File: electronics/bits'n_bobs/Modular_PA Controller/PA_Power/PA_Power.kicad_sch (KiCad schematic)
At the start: 54 parts, among them J1 Screw_Terminal_01x02, J2 Screw_Terminal_01x02, J3 Conn_01x04, J4 Conn_01x04, J5 Conn_01x04, J6 Conn_01x04, J7 Conn_01x02, Q1 Q_PMOS_DGS, Q2 Q_NMOS_DGS, U1 ACS758xCB-050U-PFF, U2 LMR38020, U3 ADS1015IDGS, U4 PCF8574A, U5 MCP4725xxx-xCH, U6 AP2204K-ADJ

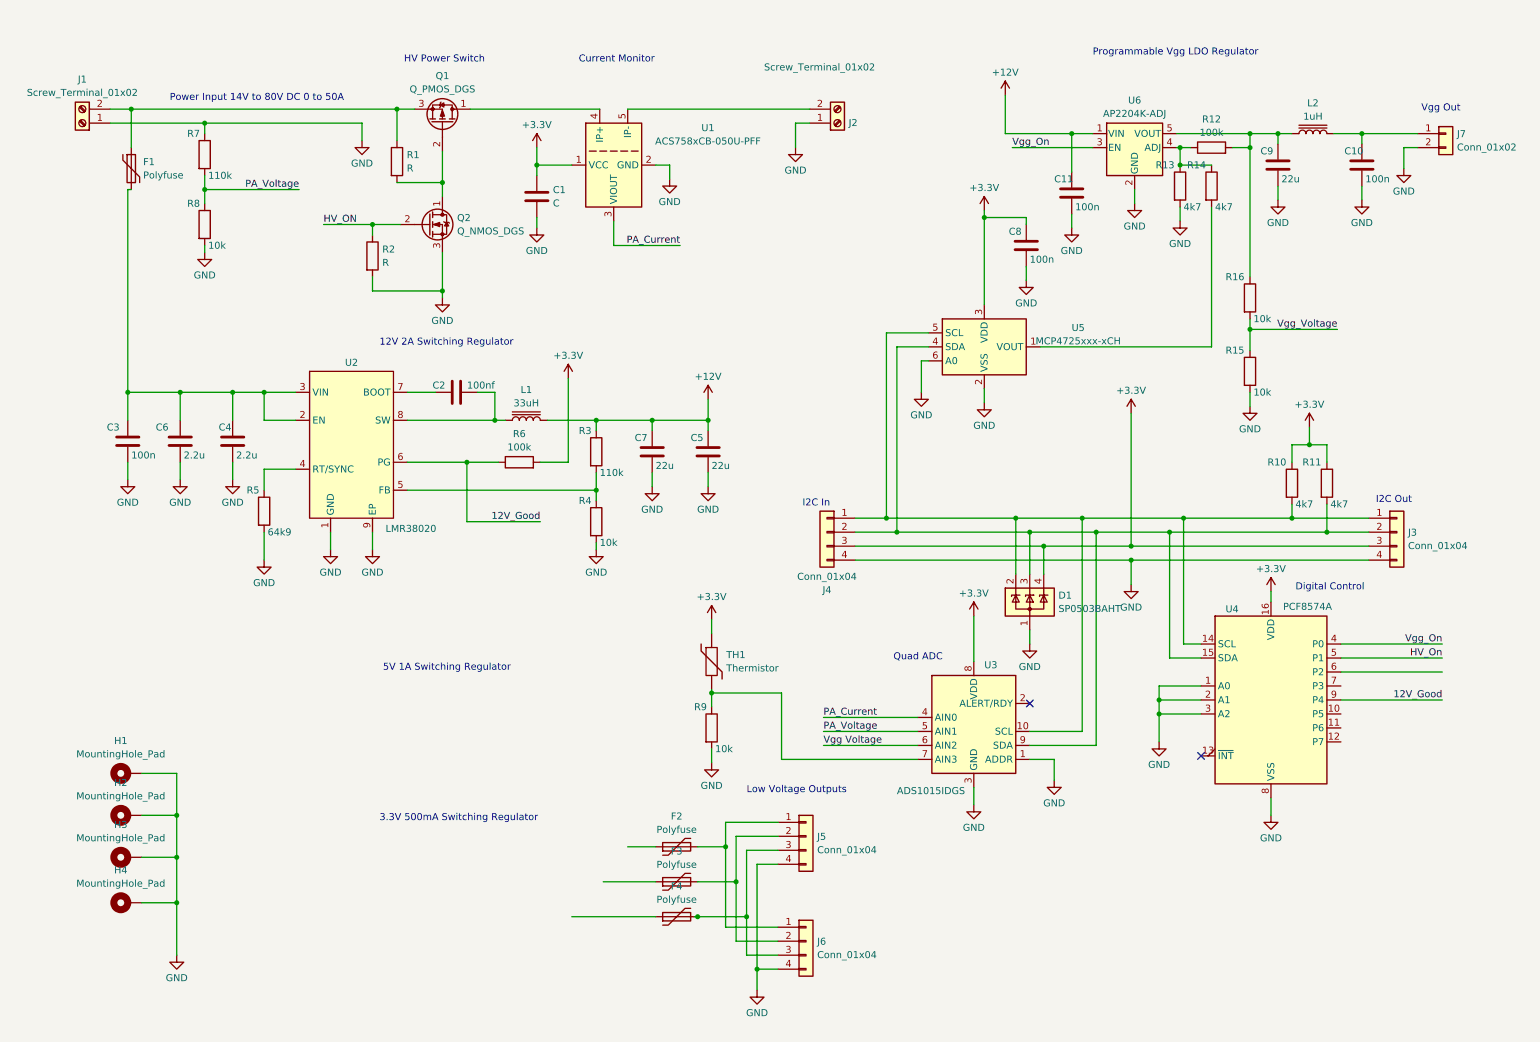
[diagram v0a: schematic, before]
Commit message: Updates in electronics bits and bobs
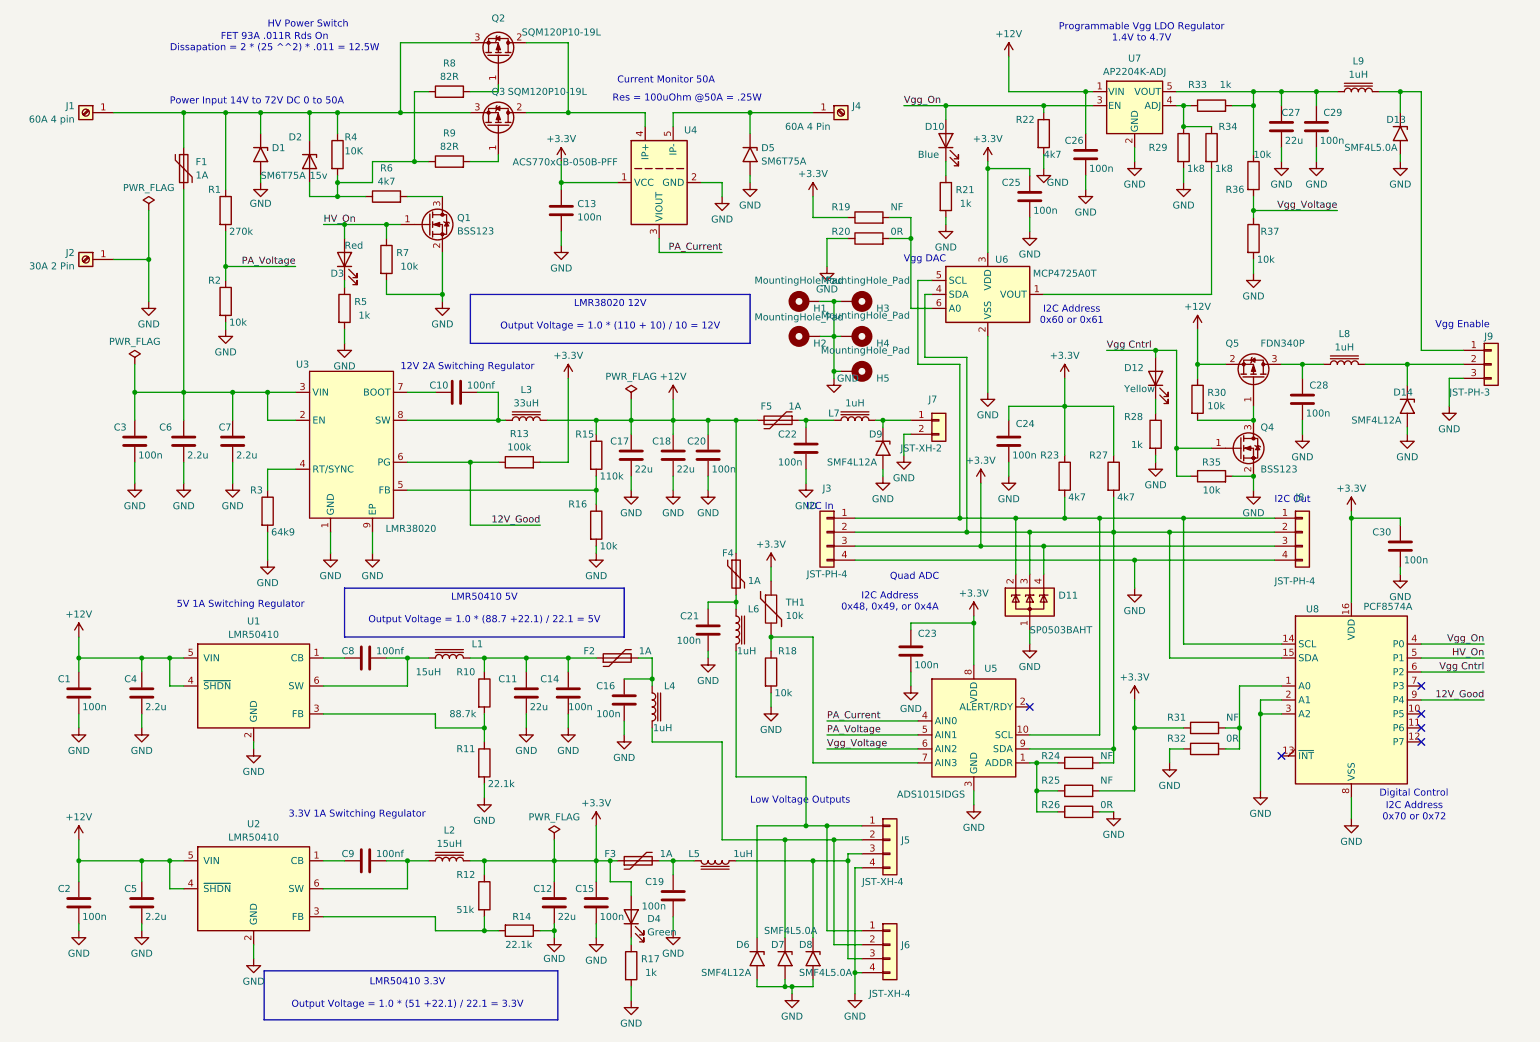
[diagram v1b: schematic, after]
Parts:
- removed J1, J2: Screw_Terminal_01x02, symbol Connector:Screw_Terminal_01x02
- removed U1: ACS758xCB-050U-PFF, Sensor_Current:Allegro_CB_PFF, symbol Sensor_Current:ACS758xCB-050U-PFF
- added C1, C14, C15, C16, C19, C2, C20, C21, C22, C23, C24, C28, C30: 100n, Capacitor_SMD:C_0603_1608Metric, symbol Device:C
- added C11, C12: 22u, Capacitor_SMD:C_1210_3225Metric, symbol Device:C
- added C4, C5: 2.2u, Capacitor_SMD:C_0603_1608Metric, symbol Device:C
- added C8, C9: 100nf, Capacitor_SMD:C_0603_1608Metric, symbol Device:C
- added D1, D5: SM6T75A, Diode_SMD:D_SMB, symbol Diode:SM6T100A
- added D10: Blue, LED_SMD:LED_0603_1608Metric, symbol Device:LED
- added D12: Yellow, LED_SMD:LED_0603_1608Metric, symbol Device:LED
- added D13, D7, D8: SMF4L5.0A, Diode_SMD:D_SOD-123F, symbol Diode:SM6T100A
- added D14, D6, D9: SMF4L12A, Diode_SMD:D_SOD-123F, symbol Diode:SM6T100A
- added D2: 15v, Diode_SMD:Nexperia_CFP3_SOD-123W, symbol Device:D_Zener
- added D3: Red, LED_SMD:LED_0603_1608Metric, symbol Device:LED
- added D4: Green, LED_SMD:LED_0603_1608Metric, symbol Device:LED
- added F5: 1A, Fuse:Fuse_1812_4532Metric, symbol Device:Polyfuse
- added H5: MountingHole_Pad, MountingHole:MountingHole_3.2mm_M3_DIN965_Pad, symbol Mechanical:MountingHole_Pad
- added J1: 60A 4 pin, PA_Control:Fat_Power 4, symbol Connector:Screw_Terminal_01x01
- added J2: 30A 2 Pin, PA_Control:Fat_Power 2, symbol Connector:Screw_Terminal_01x01
- added J4: 60A 4 Pin, PA_Control:Fat_Power 4, symbol Connector:Screw_Terminal_01x01
- added J9: JST-PH-3, Connector_JST:JST_PH_S3B-PH-SM4-TB_1x03-1MP_P2.00mm_Horizontal, symbol Connector_Generic:Conn_01x03
- added L1, L2: 15uH, Inductor_SMD:L_Wuerth_MAPI-4030, symbol Device:L_Iron
- added L4, L5, L6, L7, L8: 1uH, Inductor_SMD:L_0805_2012Metric, symbol Device:L_Iron
- added Q2: SQM120P10-19L, PA_Control:TO263_Heatsink_301, symbol Device:Q_PMOS_GDS
- added Q4: BSS123, Package_TO_SOT_SMD:SOT-23, symbol Transistor_FET:BSS123
- added Q5: FDN340P, Package_TO_SOT_SMD:SOT-23, symbol Transistor_FET:FDN340P
- added R10: 88.7k, Resistor_SMD:R_0603_1608Metric, symbol Device:R
- added R11, R14: 22.1k, Resistor_SMD:R_0603_1608Metric, symbol Device:R
- added R12: 51k, Resistor_SMD:R_0603_1608Metric, symbol Device:R
- added R17, R21, R28, R5: 1k, Resistor_SMD:R_0603_1608Metric, symbol Device:R
- added R19, R24, R25, R31: NF, Resistor_SMD:R_0603_1608Metric, symbol Device:R
- added R20, R26, R32: 0R, Resistor_SMD:R_0603_1608Metric, symbol Device:R
- added R22, R6: 4k7, Resistor_SMD:R_0603_1608Metric, symbol Device:R
- added R30, R35: 10k, Resistor_SMD:R_0603_1608Metric, symbol Device:R
- added R8, R9: 82R, Resistor_SMD:R_0603_1608Metric, symbol Device:R
- added U1, U2: LMR50410, Package_TO_SOT_SMD:SOT-23-6, symbol PA_Control:LMR50410
- added U4: ACS770xCB-050B-PFF, PA_Control:Allegro_CB_PFF, symbol Sensor_Current:ACS770xCB-050B-PFF
- C10: renamed from C2; footprint (none) -> Capacitor_SMD:C_0603_1608Metric
- C13: renamed from C1; value C -> 100n; footprint (none) -> Capacitor_SMD:C_0603_1608Metric
- C17: renamed from C7; footprint (none) -> Capacitor_SMD:C_1210_3225Metric
- C18: renamed from C5; footprint (none) -> Capacitor_SMD:C_1210_3225Metric
- C25: renamed from C8; footprint (none) -> Capacitor_SMD:C_0603_1608Metric
- C26: renamed from C11; footprint (none) -> Capacitor_SMD:C_0603_1608Metric
- C27: renamed from C9; footprint (none) -> Capacitor_SMD:C_0805_2012Metric
- C29: renamed from C10; footprint (none) -> Capacitor_SMD:C_0603_1608Metric
- C3: footprint (none) -> Capacitor_SMD:C_0805_2012Metric
- C6: footprint (none) -> Capacitor_SMD:C_1210_3225Metric
- C7: renamed from C4; footprint (none) -> Capacitor_SMD:C_1210_3225Metric
- F1: value Polyfuse -> 1A; footprint (none) -> Fuse:Fuse_Schurter_UMZ250
- F2: renamed from F3; value Polyfuse -> 1A; footprint (none) -> Fuse:Fuse_1812_4532Metric
- F3: renamed from F4; value Polyfuse -> 1A; footprint (none) -> Fuse:Fuse_1812_4532Metric
- F4: renamed from F2; value Polyfuse -> 1A; footprint (none) -> Fuse:Fuse_1812_4532Metric
- H1: renamed from H3; footprint (none) -> MountingHole:MountingHole_3.2mm_M3_DIN965_Pad
- H2: renamed from H4; footprint (none) -> MountingHole:MountingHole_3.2mm_M3_DIN965_Pad
- H3: renamed from H1; footprint (none) -> MountingHole:MountingHole_3.2mm_M3_DIN965_Pad
- H4: renamed from H2; footprint (none) -> MountingHole:MountingHole_3.2mm_M3_DIN965_Pad
- J3: renamed from J4; value Conn_01x04 -> JST-PH-4; footprint (none) -> Connector_JST:JST_PH_B4B-PH-SM4-TB_1x04-1MP_P2.00mm_Vertical
- J5, J6: value Conn_01x04 -> JST-XH-4; footprint (none) -> Connector_JST:JST_XH_S4B-XH-A_1x04_P2.50mm_Horizontal
- J7: value Conn_01x02 -> JST-XH-2; footprint (none) -> Connector_JST:JST_XH_S2B-XH-A_1x02_P2.50mm_Horizontal
- J8: renamed from J3; value Conn_01x04 -> JST-PH-4; footprint (none) -> Connector_JST:JST_PH_B4B-PH-SM4-TB_1x04-1MP_P2.00mm_Vertical
- L3: renamed from L1; footprint (none) -> Inductor_SMD:L_Coilcraft_MSS1210-XXX
- L9: renamed from L2; footprint (none) -> Inductor_SMD:L_0805_2012Metric
- Q1: renamed from Q2; value Q_NMOS_DGS -> BSS123; footprint (none) -> Package_TO_SOT_SMD:SOT-23; symbol Device:Q_NMOS_DGS -> Transistor_FET:BSS123
- Q3: renamed from Q1; value Q_PMOS_DGS -> SQM120P10-19L; footprint (none) -> PA_Control:TO263_Heatsink_301; symbol Device:Q_PMOS_DGS -> Device:Q_PMOS_GDS
- R1: renamed from R7; value 110k -> 270k; footprint (none) -> Resistor_SMD:R_0603_1608Metric
- R13: renamed from R6; footprint (none) -> Resistor_SMD:R_0603_1608Metric
- R15: renamed from R3; footprint (none) -> Resistor_SMD:R_0603_1608Metric
- R16: renamed from R4; footprint (none) -> Resistor_SMD:R_0603_1608Metric
- R18: renamed from R9; footprint (none) -> Resistor_SMD:R_0603_1608Metric
- R2: renamed from R8; footprint (none) -> Resistor_SMD:R_0603_1608Metric
- R23: renamed from R10; footprint (none) -> Resistor_SMD:R_0603_1608Metric
- R27: renamed from R11; footprint (none) -> Resistor_SMD:R_0603_1608Metric
- R29: renamed from R13; value 4k7 -> 1k8; footprint (none) -> Resistor_SMD:R_0603_1608Metric
- R3: renamed from R5; footprint (none) -> Resistor_SMD:R_0603_1608Metric
- R33: renamed from R12; value 100k -> 1k; footprint (none) -> Resistor_SMD:R_0603_1608Metric
- R34: renamed from R14; value 4k7 -> 1k8; footprint (none) -> Resistor_SMD:R_0603_1608Metric
- R36: renamed from R16; footprint (none) -> Resistor_SMD:R_0603_1608Metric
- R37: renamed from R15; footprint (none) -> Resistor_SMD:R_0603_1608Metric
- R4: renamed from R1; value R -> 10K; footprint (none) -> Resistor_SMD:R_0603_1608Metric
- R7: renamed from R2; value R -> 10k; footprint (none) -> Resistor_SMD:R_0603_1608Metric
- TH1: value Thermistor -> 10k; footprint (none) -> Resistor_SMD:R_0603_1608Metric
- U3: renamed from U2; footprint (none) -> PA_Control:lmr38012
- U6: renamed from U5; value MCP4725xxx-xCH -> MCP4725A0T
- U8: renamed from U4; footprint (none) -> Package_SO:SOIC-16W_7.5x10.3mm_P1.27mm
- renumbered D1 to D11, U3 to U5, U6 to U7
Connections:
- net Vgg Voltage is gone; now on net Vgg_Voltage: U5.6 (AIN2)
- net +12V: now also F4.1, C1.1, C2.1, C20.1, C4.1, C5.1, F5.2, Q5.2 (S), R30.1, U1.4 (~{SHDN}), U1.5 (VIN), U2.4 (~{SHDN}), U2.5 (VIN)
- net +3.3V: now also F3.1, C12.1, C15.1, C23.1, C24.1, C30.1, D4.2 (A), L2.2, R12.1, R19.1, R25.2, R31.1, U4.1 (VCC)
- net GND: now also Q1.2 (S), C1.2, C11.2, C12.2, C14.2, C15.2, C16.2, C19.2, C2.2, C20.2, C21.2, C22.2, C23.2, C24.2, C28.2, C30.2, C4.2, C5.2, D1.2 (A2), D13.2 (A2), D14.2 (A2), D5.2 (A2), D6.2 (A2), D7.2 (A2), D8.2 (A2), D9.2 (A2), H5.1, J2.1 (Pin_1), J9.3 (Pin_3), Q4.2 (S), R11.2, R14.1, R17.2, R20.1, R21.2, R22.2, R26.2, R28.2, R32.1, R35.2, R5.2, U1.2 (GND), U2.2 (GND), U4.2 (GND); no longer Q1.3 (S), R1.1, U5.1 (ADDR), U6.6 (A0), U8.1 (A0)
- net HV_On: now also Q1.1 (G), R7.1, D3.2 (A)
- net PA_Current: now also U4.3 (VIOUT)
- net Vgg_On: now also D10.2 (A), R22.1
- net at C27.1, L9.1, R33.2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: now also C29.1
- net at J5.1 (Pin_1), J6.1 (Pin_1): now also D6.1 (A1), L6.2; no longer F4.2
- net at D11.3 (K), J3.2 (Pin_2), J8.2 (Pin_2)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: now also R24.2
- net at F2.1: now also C11.1, C14.1, L1.2, R10.1
- net at J5.2 (Pin_2), J6.2 (Pin_2): now also D7.1 (A1), L4.2; no longer F2.2
- net at F1.1, Q3.3 (S), R4.1: now also R1.1, D1.1 (A1), D2.1 (K), J1.1 (Pin_1), Q2.3 (S)
- net Vgg Cntrl: now reaches U8.6 (P2)
- net Vgg Cntrl: now also D12.2 (A), Q4.1 (G), R35.1
- net at J5.3 (Pin_3), J6.3 (Pin_3): now also D8.1 (A1), L5.1; no longer F3.2
- net at Q3.1 (G): now also R9.2
- removed net HV_ON: Q1.2 (G), R7.1
- new net: C21.1, F4.2, L6.1
- new net: R24.1, R25.1, R26.1, U5.1 (ADDR)
- new net: R19.2, R20.2, U6.6 (A0)
- new net: Q4.3 (D), Q5.1 (G), R30.2
- new net: C16.1, F2.2, L4.1
- new net: C8.2, L1.1, U1.6 (SW)
- new net: D2.2 (A), R4.2, R6.1, R8.1, R9.1
- new net: D9.1 (A1), J7.1 (Pin_1), L7.2
- new net: D3.1 (K), R5.1
- new net: C22.1, F5.1, L7.1
- new net: R12.2, R14.2, U2.3 (FB)
- new net: D14.1 (A1), J9.2 (Pin_2), L8.2
- new net: D13.1 (A1), J9.1 (Pin_1), L9.2
- new net: C8.1, U1.1 (CB)
- new net: C9.2, L2.1, U2.6 (SW)
- new net: C28.1, L8.1, Q5.3 (D)
- new net: D5.1 (A1), J4.1 (Pin_1), U4.5 (IP-)
- new net: D4.1 (K), R17.1
- new net: C9.1, U2.1 (CB)
- new net: Q2.2 (D), Q3.2 (D), U4.4 (IP+)
- new net: R31.2, R32.2, U8.1 (A0)
- new net: D12.1 (K), R28.1
- new net: C19.1, F3.2, L5.2
- new net: Q2.1 (G), R8.2
- new net: R10.2, R11.1, U1.3 (FB)
- new net: Q1.3 (D), R6.2
- new net: D10.1 (K), R21.1
- no-connect marks 2 -> 6
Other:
- note added: "3.3V 1A Switching Regulator"
- note added: "Current Monitor 50A"
- note added: "FET 93A .011R Rds On Dissapation = 2 * (25 ^^2) * .011 = 12.5W"
- note added: "I2C Address 0x48, 0x49, or 0x4A"
- note added: "I2C Address 0x60 or 0x61"
- note added: "I2C Address 0x70 or 0x72"
- note added: "LMR38020 12V Output Voltage = 1.0 * (110 + 10) / 10 = 12V"
- note added: "LMR50410 3.3V Output Voltage = 1.0 * (51 +22.1) / 22.1 = 3.3V"
- note added: "LMR50410 5V Output Voltage = 1.0 * (88.7 +22.1) / 22.1 = 5V"
- note added: "Power Input 14V to 72V DC 0 to 50A"
- note added: "Programmable Vgg LDO Regulator 1.4V to 4.7V"
- note added: "Res = 100uOhm @50A = .25W"
- note added: "Vgg DAC"
- note added: "Vgg Enable"
- note removed: "3.3V 500mA Switching Regulator"
- note removed: "Current Monitor"
- note removed: "Power Input 14V to 80V DC 0 to 50A"
- note removed: "Programmable Vgg LDO Regulator"
- note removed: "Vgg Out"
- moved on the sheet: C13, C17, C18, C25, C26, C27, C29, C3, C6, F1, F2, F3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
